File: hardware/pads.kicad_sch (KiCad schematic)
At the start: 56 parts, among them J1 5V, J10 5V, J11 5V, J12 5V, J13 5V, J14 5V, J15 5V, J16 5V, J17 5V, J18 5V, J19 5V, J2 5V, J20 5V, J21 5V, J22 5V, J23 5V, J24 5V, J25 5V, J26 5V, J27 5V, J28 5V, J29 5V, J3 5V, J30 5V, J31 5V, J32 5V, J33 5V, J34 5V, J35 5V, J36 5V, J37 5V, J38 5V, J39 5V, J4 5V, J40 5V, J41 5V, J42 5V, J43 5V, J44 5V, J45 5V, J46 5V, J47 5V, J48 5V, J49 5V, J5 5V, J50 5V, J51 5V, J52 5V, J53 5V, J54 5V, J6 5V, J7 5V, J8 5V, J9 5V, P1 SM08B-SRSS-TB(LF)(SN), U8 SM06B-SRSS-TB(LF)(SN)

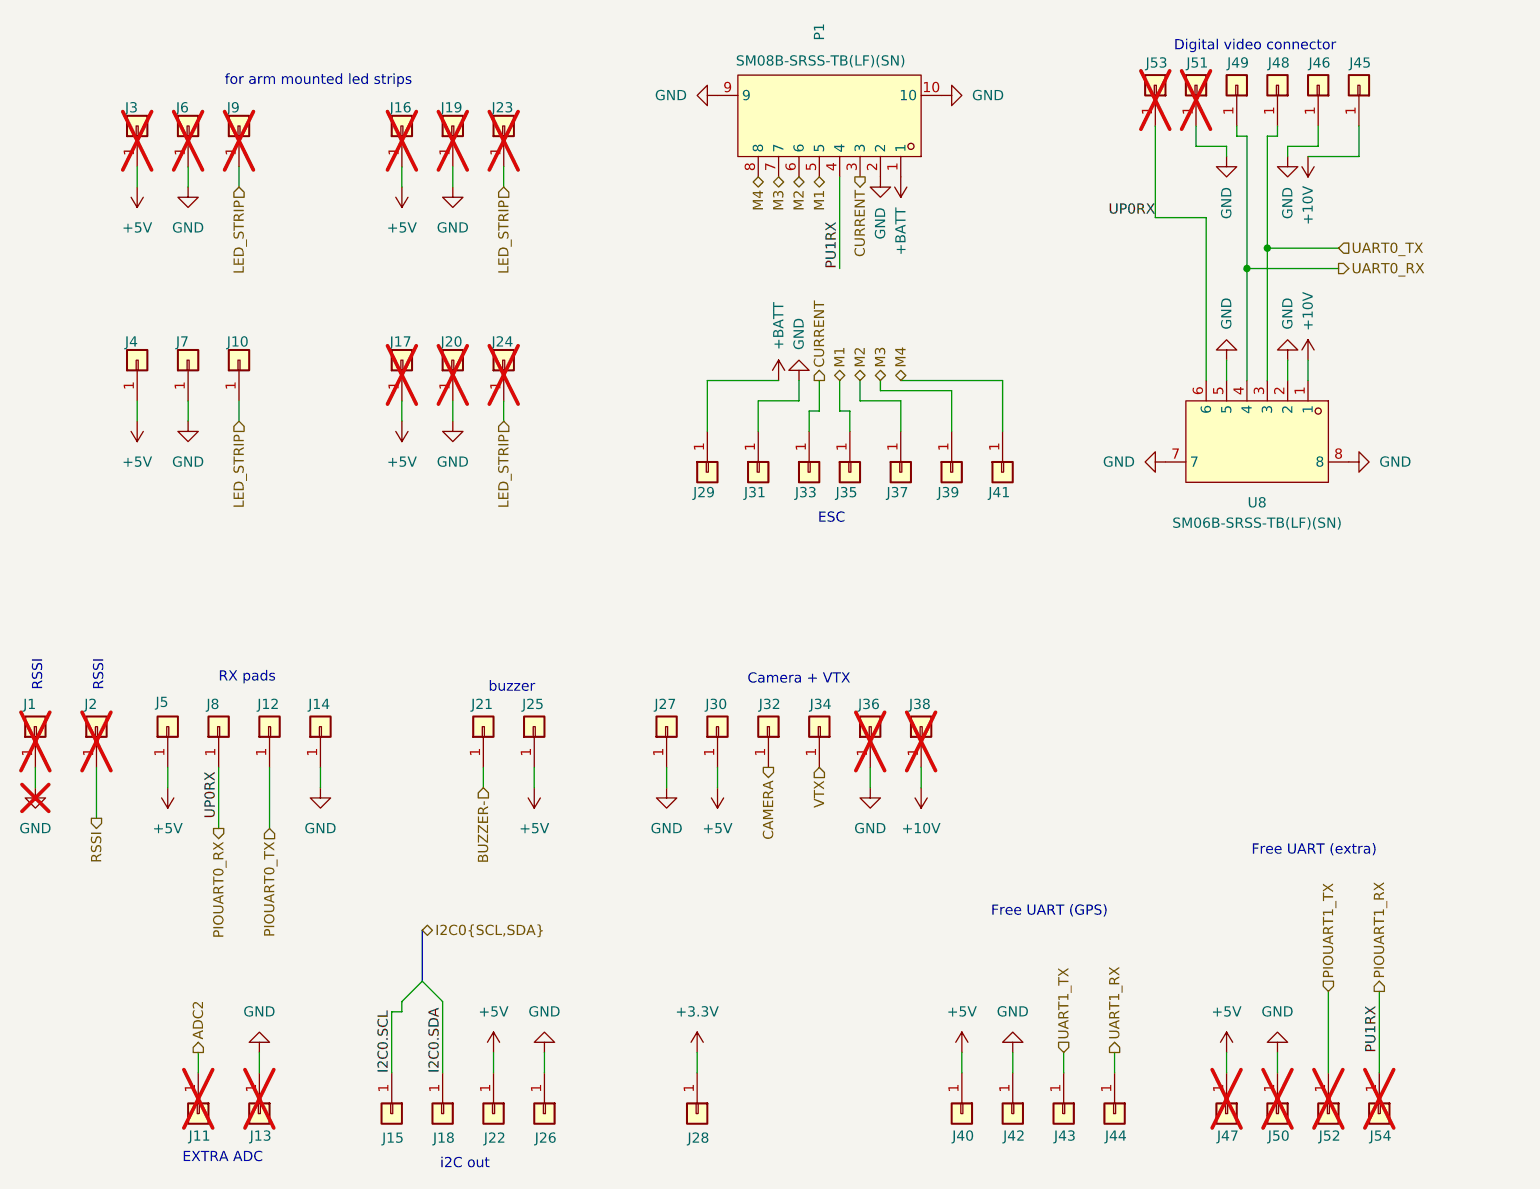
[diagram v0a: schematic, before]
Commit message: piu1
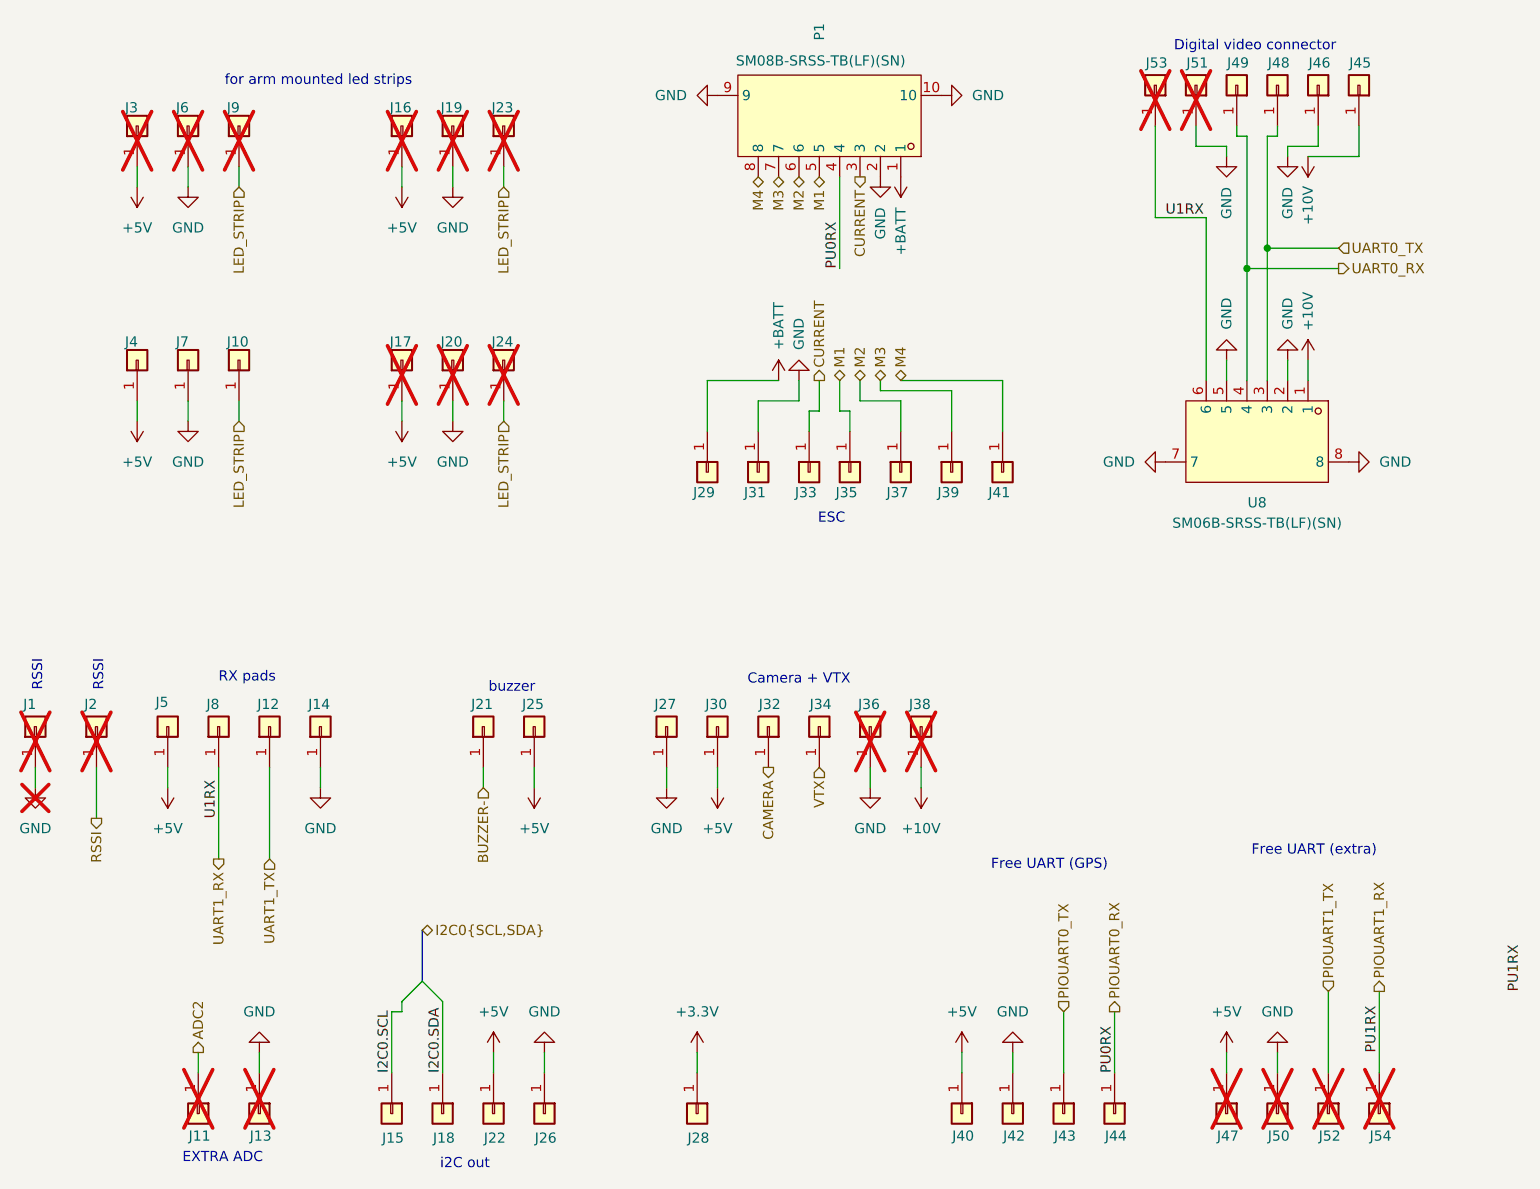
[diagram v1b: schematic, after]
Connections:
- net PIOUART0_RX: now also J44.1 (Pin_1), P1.4; no longer J53.1 (Pin_1), J8.1 (Pin_1), U8.6
- net PIOUART0_TX: now also J43.1 (Pin_1); no longer J12.1 (Pin_1)
- net PIOUART1_RX: no longer P1.4
- net UART1_RX: now also J53.1 (Pin_1), J8.1 (Pin_1), U8.6; no longer J44.1 (Pin_1)
- net UART1_TX: now also J12.1 (Pin_1); no longer J43.1 (Pin_1)
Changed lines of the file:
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@@
 	(text "Free UART (GPS)"
 		(exclude_from_sim no)
-		(at 159.512 125.984 0)
+		(at 159.512 120.142 0)
 		(effects
 			(font
@@
 	(wire
 		(pts
-			(xy 161.29 146.05) (xy 161.29 143.51)
+			(xy 161.29 146.05) (xy 161.29 138.43)
 		)
 		(stroke
@@
 	(wire
 		(pts
-			(xy 55.88 107.95) (xy 55.88 115.57)
-		)
-		(stroke
-			(width 0)
-			(type default)
-		)
-	)
-	(wire
-		(pts
 			(xy 115.57 146.05) (xy 115.57 143.51)
 		)
@@
 	(wire
 		(pts
-			(xy 62.23 107.95) (xy 62.23 115.57)
+			(xy 62.23 107.95) (xy 62.23 119.38)
 		)
 		(stroke
@@
 	(wire
 		(pts
+			(xy 55.88 107.95) (xy 55.88 119.38)
+		)
+		(stroke
+			(width 0)
+			(type default)
+		)
+	)
+	(wire
+		(pts
 			(xy 187.96 146.05) (xy 187.96 143.51)
 		)
@@
 	(wire
 		(pts
-			(xy 167.64 146.05) (xy 167.64 143.51)
+			(xy 167.64 146.05) (xy 167.64 138.43)
 		)
 		(stroke
@@
 		)
 	)
-	(label "UP0RX"
-		(at 172.72 39.37 180)
-		(effects
-			(font
-				(size 1.27 1.27)
-			)
-			(justify right bottom)
-		)
-	)
-	(label "UP0RX"
+	(label "PU0RX"
+		(at 167.64 146.05 90)
+		(effects
+			(font
+				(size 1.27 1.27)
+			)
+			(justify left bottom)
+		)
+	)
+	(label "PU0RX"
+		(at 133.35 45.72 90)
+		(effects
+			(font
+				(size 1.27 1.27)
+			)
+			(justify left bottom)
+		)
+	)
+	(label "U1RX"
 		(at 55.88 114.3 90)
+		(effects
+			(font
+				(size 1.27 1.27)
+			)
+			(justify left bottom)
+		)
+	)
+	(label "PU1RX"
+		(at 218.44 135.89 90)
 		(effects
 			(font
@@
 		)
 	)
-	(label "PU1RX"
-		(at 133.35 45.72 90)
+	(label "U1RX"
+		(at 173.99 39.37 0)
 		(effects
 			(font
@@
 	(hierarchical_label "PIOUART0_TX"
 		(shape input)
-		(at 62.23 115.57 270)
-		(effects
-			(font
-				(size 1.27 1.27)
-			)
-			(justify right)
+		(at 161.29 138.43 90)
+		(effects
+			(font
+				(size 1.27 1.27)
+			)
+			(justify left)
 		)
 	)
@@
 	(hierarchical_label "PIOUART0_RX"
 		(shape output)
-		(at 55.88 115.57 270)
-		(effects
-			(font
-				(size 1.27 1.27)
-			)
-			(justify right)
+		(at 167.64 138.43 90)
+		(effects
+			(font
+				(size 1.27 1.27)
+			)
+			(justify left)
 		)
 	)
@@
 	(hierarchical_label "UART1_RX"
 		(shape output)
-		(at 167.64 143.51 90)
-		(effects
-			(font
-				(size 1.27 1.27)
-			)
-			(justify left)
+		(at 55.88 119.38 270)
+		(effects
+			(font
+				(size 1.27 1.27)
+			)
+			(justify right)
 		)
 	)
@@
 	(hierarchical_label "UART1_TX"
 		(shape input)
-		(at 161.29 143.51 90)
-		(effects
-			(font
-				(size 1.27 1.27)
-			)
-			(justify left)
-		)
-	)
+		(at 62.23 119.38 270)
+		(effects
+			(font
+				(size 1.27 1.27)
+			)
+			(justify right)
+		)
+	)

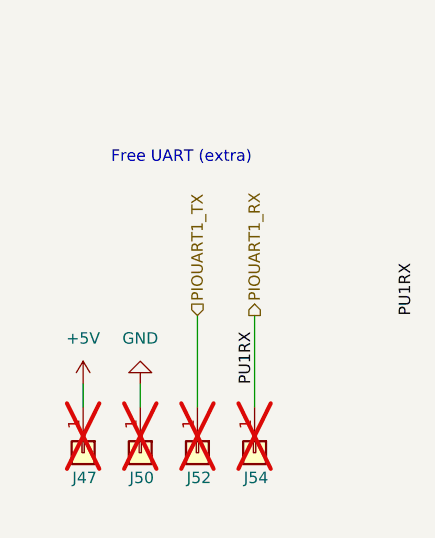
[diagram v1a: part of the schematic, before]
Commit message: switch spi
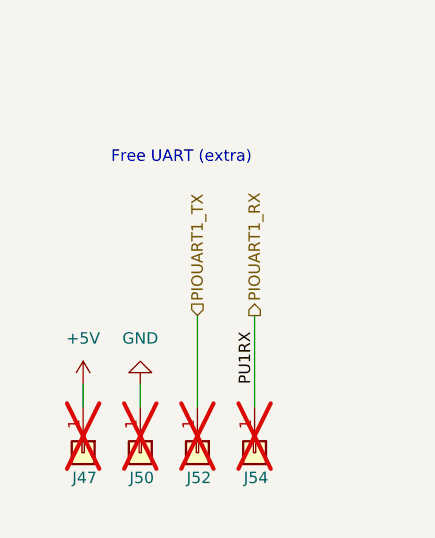
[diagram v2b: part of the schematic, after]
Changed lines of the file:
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@@
-		)
-	)
-	(label "PU1RX"
-		(at 218.44 135.89 90)
-		(effects
-			(font
-				(size 1.27 1.27)
-			)
-			(justify left bottom)
 		)
 	)
